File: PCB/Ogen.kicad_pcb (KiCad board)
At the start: 2 copper layers, 28 x 21.5 mm, 17 parts, among them J1 Input, U1 PMW3360DM-T2QU, U2 TLV70019, U3 TXS0102DCU, U4 TXS0102DCU, U5 TXS0102DCU

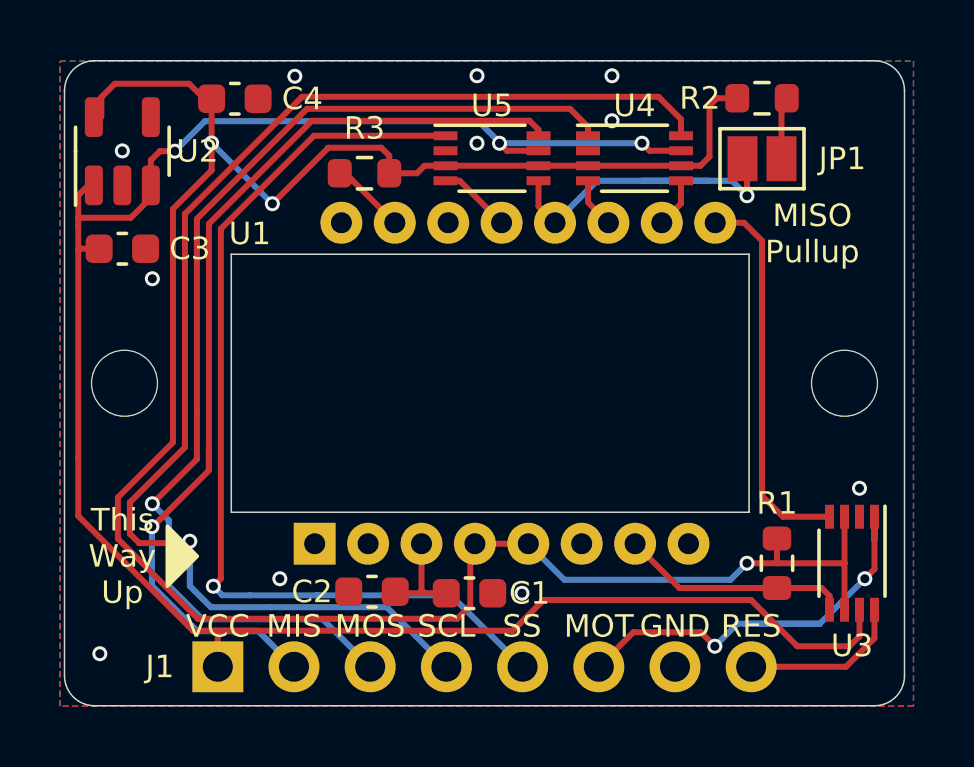
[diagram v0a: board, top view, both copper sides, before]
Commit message: V1.2 update.
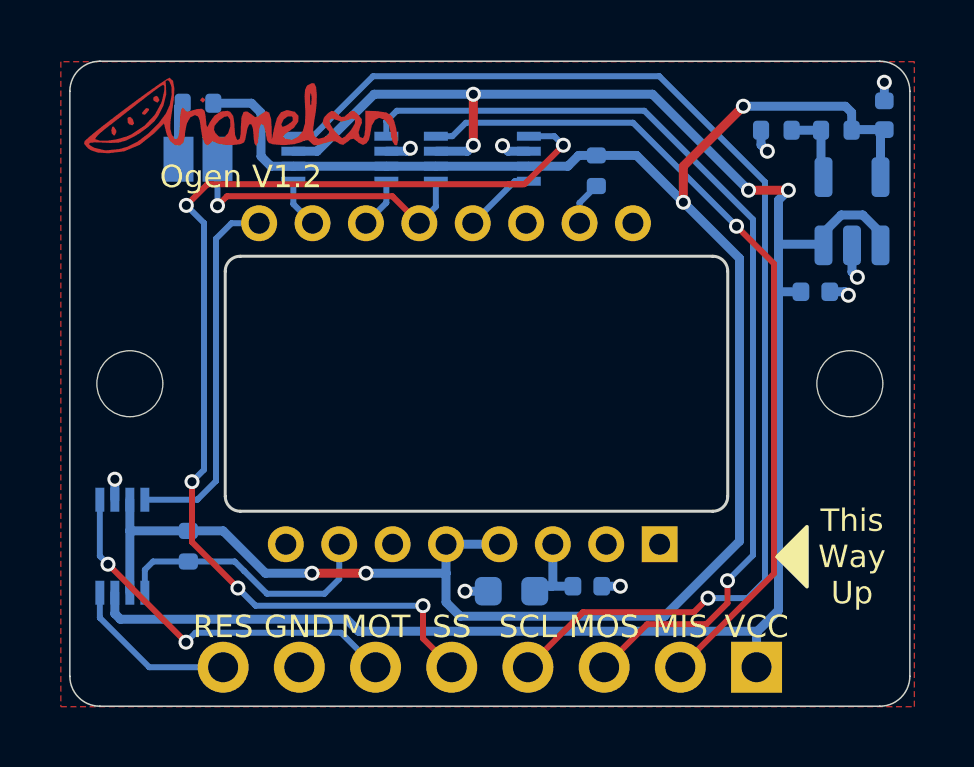
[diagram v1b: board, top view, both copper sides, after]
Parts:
- added R4: 10k, Resistor_SMD:R_0402_1005Metric, B.Cu at (36.3, 15.3)
- added R5: 15k, Resistor_SMD:R_0402_1005Metric, B.Cu at (38.3, 15.3)
- A1: footprint Ogen:Ariamelon_Logo -> Ogen:Ariamelon_Logo-CU; moved to F.Cu
- C1: value 4.7uF -> 4u7; moved to B.Cu
- C2: value 100nF -> 100n; footprint Capacitor_SMD:C_0603_1608Metric -> Capacitor_SMD:C_0402_1005Metric; moved to B.Cu
- C3, C4: value 1uF -> 1u; footprint Capacitor_SMD:C_0603_1608Metric -> Capacitor_SMD:C_0402_1005Metric; moved to B.Cu
- H1, H2, J1, JP1, U1, U3, U4, U5: moved to B.Cu
- R1, R2: footprint Resistor_SMD:R_0603_1608Metric -> Resistor_SMD:R_0402_1005Metric; moved to B.Cu
- R3: value 39R -> 39; footprint Resistor_SMD:R_0603_1608Metric -> Resistor_SMD:R_0402_1005Metric; moved to B.Cu
- U2: value TLV70019 -> AP2127K-ADJ; moved to B.Cu
- moved U2 24.4 mm to (38.8, 18.0)
- moved U3 24.3 mm to (14.5, 29.2)
- moved H1 24.2 mm to (38.7, 23.8)
- moved H2 23.8 mm to (14.8, 23.7)
- moved C3 23.1 mm to (37.6, 20.7)
- moved C4 21.7 mm to (39.9, 14.8), turned to 90 degrees
- moved R1 19.6 mm to (16.7, 29.2)
- moved R2 18.8 mm to (17.0, 14.4)
- moved JP1 18.8 mm to (17.0, 16.3), turned to 0 degrees
- moved U4 9.82 mm to (21.8, 16.2), turned to 180 degrees
- moved A1 8.89 mm to (18.4, 14.8), turned to 0 degrees
- moved R3 7.73 mm to (30.3, 16.6), turned to 90 degrees
- moved C2 7.18 mm to (30.0, 30.5)
- moved C1 1.40 mm to (27.5, 30.7), turned to 180 degrees
- moved U5 0.32 mm to (26.5, 16.2), turned to 180 degrees
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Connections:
- C1 pad 1: Net-(C1-Pad1) -> Net-(U1-VDDPIX)
- C2 pad 1: Net-(C1-Pad1) -> GND
- C2 pad 2: GND -> Net-(U1-VDDPIX)
- C4 pad 1: VDD -> +2V
- JP1 pad 1: Net-(JP1-Pad1) -> Net-(JP1-A)
- R1 pad 2: VDD -> +2V
- R2 pad 1: Net-(JP1-Pad1) -> +2V
- R2 pad 2: VDD -> Net-(JP1-A)
- R3 pad 2: VDD -> +2V
- U1 pad 3: Net-(C1-Pad1) -> Net-(U1-VDDPIX)
- U1 pad 4: VDD -> +2V
- U1 pad 5: VDD -> +2V
- U2 pad 4: unconnected-(U2-Pad4) -> Net-(U2-ADJ)
- U2 pad 5: VDD -> +2V
- U3 pad 3: VDD -> +2V
- U3 pad 6: VDD -> +2V
- U4 pad 3: VDD -> +2V
- U4 pad 6: VDD -> +2V
- U5 pad 3: VDD -> +2V
- U5 pad 6: VDD -> +2V
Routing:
- net VDD: track 74.4 -> 0.00 mm, vias 3 -> 0
- net +2V: track 0.00 -> 70.2 mm, vias 0 -> 4
- net GND: track 0.00 -> 7.09 mm, vias 11 -> 9
- net MISO-H: track 34.3 -> 28.1 mm
- net SS-H: track 32.2 -> 37.8 mm, vias 1 -> 5
- net VCC: track 70.0 -> 65.9 mm, vias 3 -> 4
- net MOSI-H: track 36.0 -> 32.5 mm
- net Net-(C1-Pad1): track 3.39 -> 0.00 mm
- net SCLK-H: track 43.8 -> 40.4 mm
- net MOT-H: track 16.0 -> 12.9 mm
- net Net-(U1-VDDPIX): track 0.00 -> 2.76 mm
- net Net-(U2-ADJ): track 0.00 -> 2.58 mm
- net Net-(JP1-Pad1): track 2.07 -> 0.00 mm
- net MISO: track 12.4 -> 10.4 mm
- net Net-(JP1-A): track 0.00 -> 1.92 mm
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- removed copper zone on B.Cu, net GND
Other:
- board text added: "Ogen V1.2"
- board text removed: "Ogen V1.1"
